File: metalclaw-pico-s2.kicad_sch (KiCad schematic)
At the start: 63 parts, among them J1 USB_C_Receptacle_USB2.0_14P, J2 Conn_01x05, J3 Conn_02x05_Odd_Even, U1 ESP32-S2, U2 MX25L3236FM2I-08G-TR, U3 APS6404L-3SQRx-SN, U5 XC6220B331MR, Y1 XRCGB40M000F1S2FR0

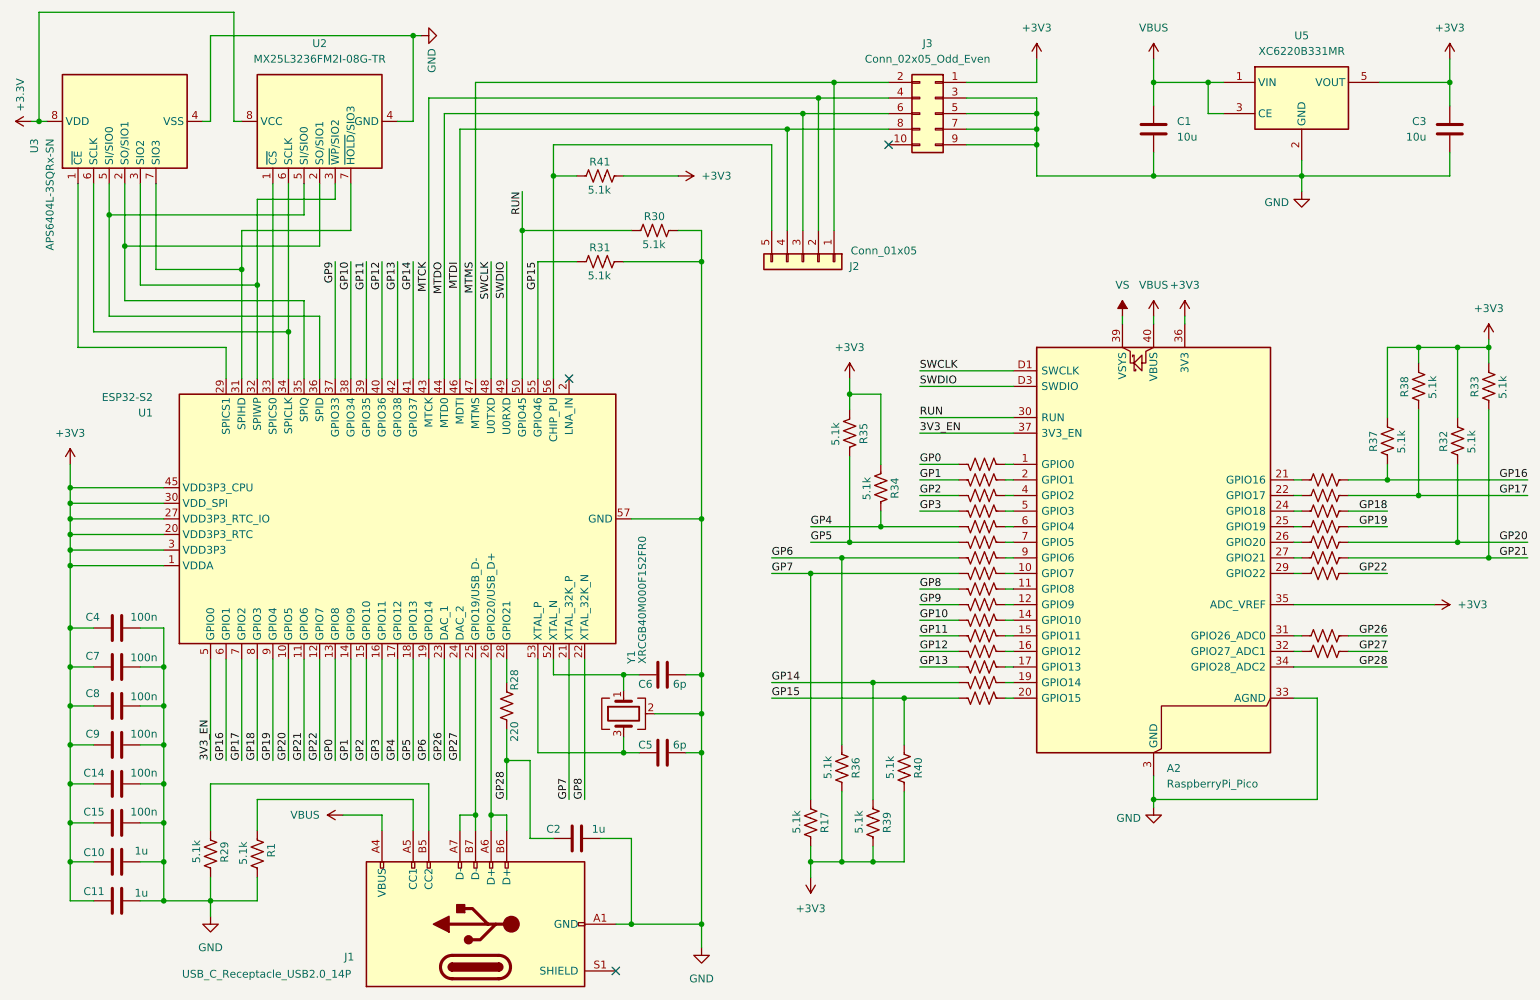
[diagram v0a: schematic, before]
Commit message: Refine schematic and layout more
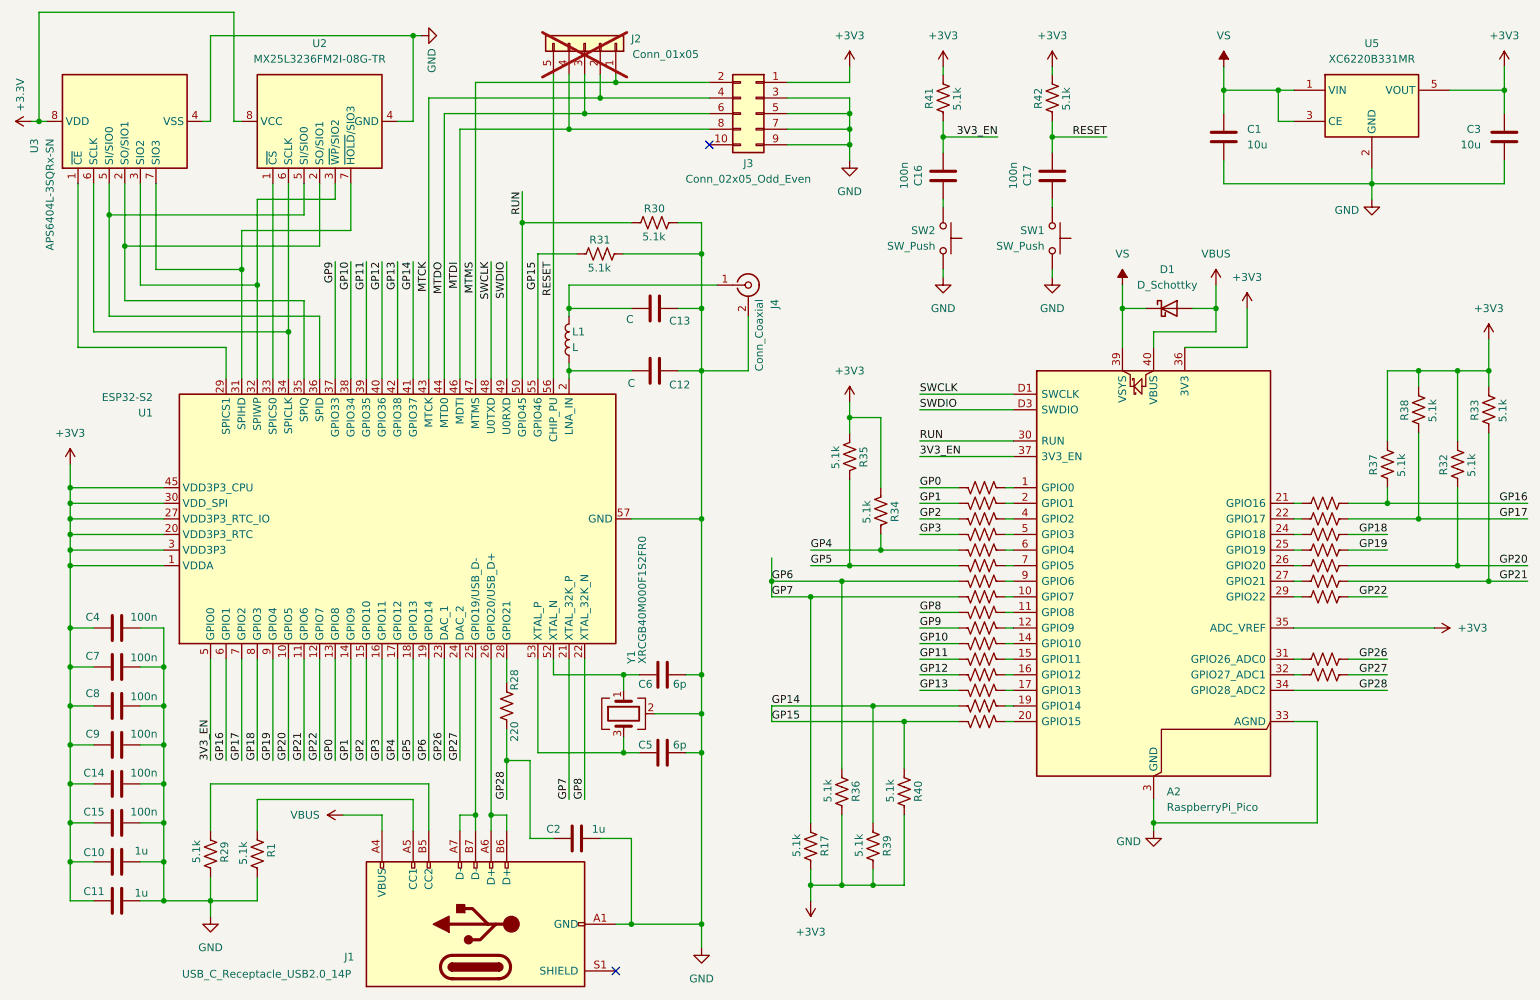
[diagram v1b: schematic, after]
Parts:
- added C12, C13: C, Capacitor_SMD:C_0402_1005Metric, symbol Device:C
- added C16, C17: 100n, Capacitor_SMD:C_0402_1005Metric, symbol Device:C
- added D1: D_Schottky, symbol Device:D_Schottky
- added J4: Conn_Coaxial, Connector_Coaxial:U.FL_Hirose_U.FL-R-SMT-1_Vertical, symbol Connector:Conn_Coaxial
- added L1: L, Inductor_SMD:L_0402_1005Metric, symbol Device:L
- added R42: 5.1k, Resistor_SMD:R_0402_1005Metric, symbol Device:R_US
- added SW1, SW2: SW_Push, Button_Switch_SMD:SW_Push_SPST_NO_Alps_SKRK, symbol Switch:SW_Push
- J2: now not fitted
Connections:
- net GP15 is gone; now on net GP14: R27.2, R31.2, R40.2, U1.55 (GPIO46)
- net GP7 is gone; now on net GP6: R17.2, R19.2, U1.21 (XTAL_32K_P)
- net +3V3: now also R42.1
- net 3V3_EN: now also R41.2, C16.2
- net GND: now also C12.2, C13.2, J4.2 (Ext), SW1.1, SW2.1
- net VBUS: now also D1.2 (A); no longer C1.1, U5.1 (VIN), U5.3 (CE)
- net VS: now also C1.1, U5.1 (VIN), U5.3 (CE), D1.1 (K)
- net RESET: now reaches J2.5 (Pin_5), U1.56 (CHIP_PU)
- net RESET: now also C17.2, R42.2; no longer R41.2
- net at U1.2 (LNA_IN): now also C12.1, L1.1
- new net: C13.1, J4.1 (In), L1.2
- new net: C17.1, SW1.2
- new net: C16.1, SW2.2
- no-connect marks 3 -> 2
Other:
- moved on the sheet: A2, C1, C3, J3, R17, R30, R31, R32, R33, R34, R35, R36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
